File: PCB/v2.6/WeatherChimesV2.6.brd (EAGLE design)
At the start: 99.3 x 79 mm, 31 parts, among them U1 MS5803-02BA, X4 BQ24074

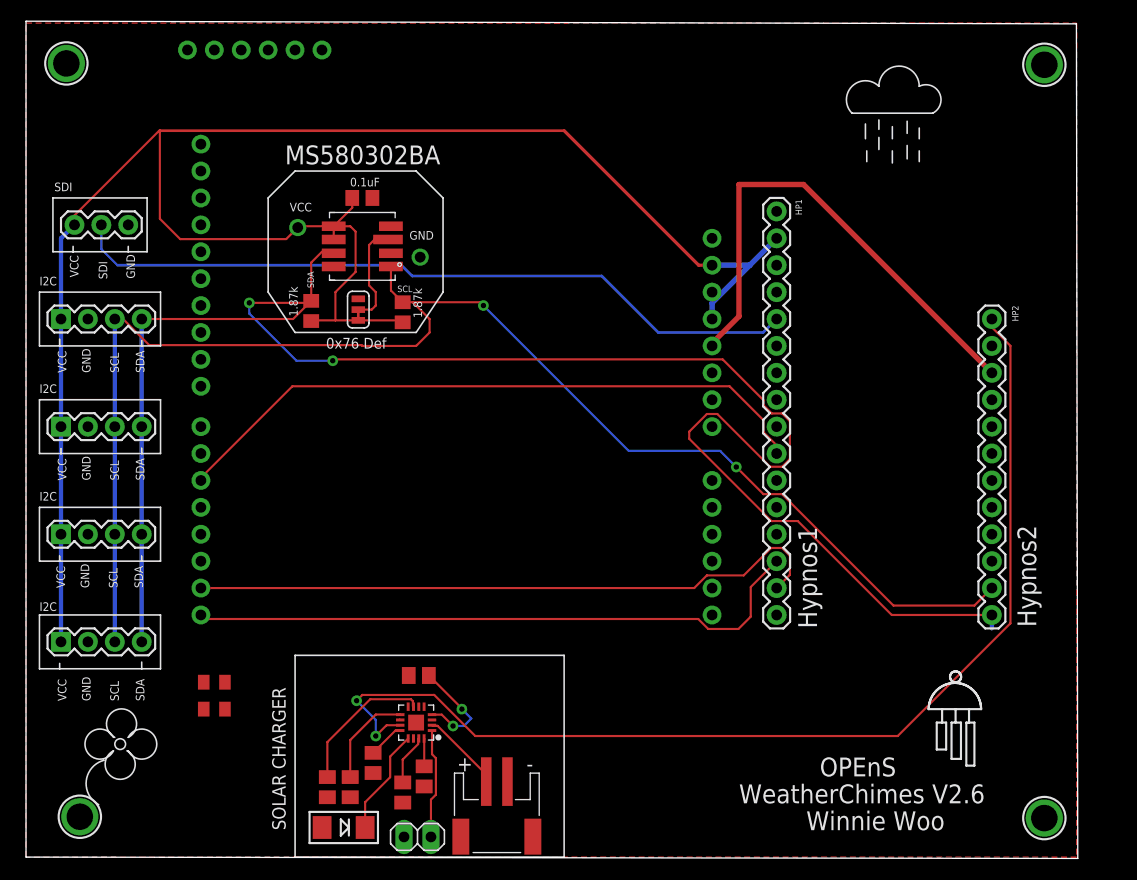
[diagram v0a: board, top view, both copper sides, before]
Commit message: WeatherChimesv2.6 files from Google Drive
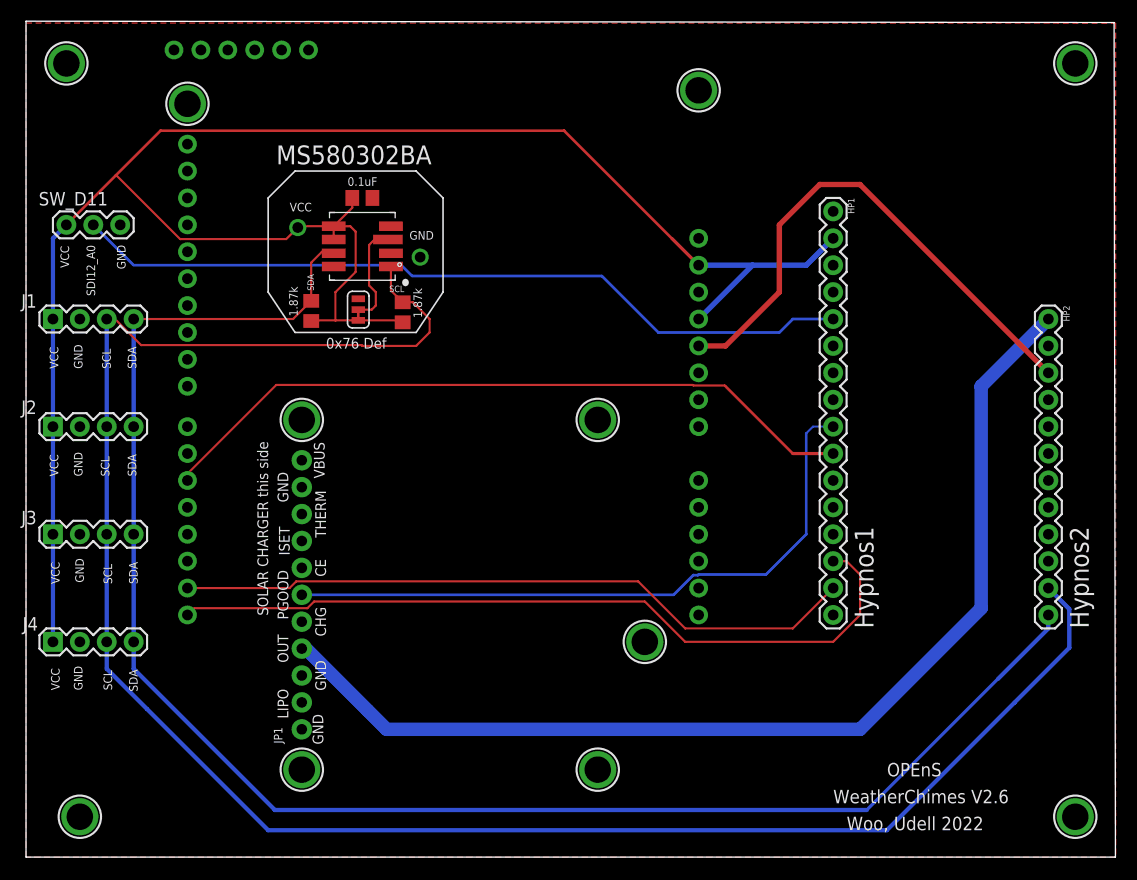
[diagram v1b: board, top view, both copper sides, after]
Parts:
- removed BATT: JST 2PH, adafruit:JST-PH-2-SMT-RA
- removed C5, C6: 10uF, adafruit:C0805K
- removed D2: SK34A, microbuilder:SMADIODE
- removed JP8: (no value), pinhead:1X02
- removed R11, R4, R7, R8: 10K, adafruit:M0805
- removed R3, R9: 1K, adafruit:M0805
- removed X4: BQ24074, adafruit_power:QFN16_3MM
- added JP1: (no value), microbuilder:1X11_ROUND_76
- added U$13, U$14, U$15, U$16, U$6, U$7, U$8: MOUNTINGHOLE2.5, microbuilder:MOUNTINGHOLE_2.5_PLATED
- moved HP1 5.33 mm to (74.9, 62.2)
- moved HP2 5.33 mm to (95.2, 52.1)
- moved U$4 2.92 mm to (97.8, 76.2)
- moved U$5 2.92 mm to (97.8, 5.08)
- moved U$1 1.27 mm to (62.2, 59.7)
- moved J1 0.76 mm to (1.27, 52.1)
- moved J2 0.76 mm to (1.27, 41.9)
- moved J3 0.76 mm to (1.27, 31.8)
- moved J4 0.76 mm to (1.27, 21.6)
- moved SW_D11 0.76 mm to (2.54, 61.0)
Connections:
- removed net !CE: R8.1, X4.4
- removed net !CHG: R7.1, X4.9
- removed net !PGOOD: R11.1, X4.7
- removed net CHARGER_IN: D2.A
- removed net ILIM: R3.1, X4.12
- removed net ISET: R9.1, X4.16
- removed net ITERM: R4.1, X4.15
- removed net N$1: X4.5
- removed net N$2: D2.C, X4.13
- removed net THERM: JP8.1, X4.1
- removed net VLIPO: BATT.1, X4.2, X4.3
- net GND: now also JP1.1, JP1.10, JP1.3; no longer BATT.2, JP8.2, R3.2, R4.2, R8.2, R9.2, X4.14, X4.6, X4.8, X4.THERMAL
- net PGOOD: now also JP1.6
- net VBAT: now also JP1.4; no longer X4.10, X4.11
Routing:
- net PGOOD: track 0.00 -> 62.3 mm
- net SCL: track 137.3 -> 184.2 mm, vias 2 -> 0
- net RX: track 58.7 -> 73.5 mm
- net !PGOOD: track 13.7 -> 0.00 mm
- net SDA: track 169.5 -> 157.0 mm, vias 2 -> 0
- net THERM: track 10.4 -> 0.00 mm
- net !CE: track 10.2 -> 0.00 mm, vias 2 -> 0
- net N$2: track 10.1 -> 0.00 mm
- net !CHG: track 9.76 -> 0.00 mm
- net VLIPO: track 7.72 -> 0.00 mm
- net 4GONOFF: track 62.7 -> 67.7 mm
- net ITERM: track 4.78 -> 0.00 mm
- net SDI: track 70.6 -> 74.6 mm
- net VCC: track 174.2 -> 177.9 mm
- net TX: track 61.0 -> 64.6 mm
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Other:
- board size 99.3 x 79 mm -> 102.8 x 78.9 mm
- board text added: "CE"
- board text added: "CHG"
- board text added: "ISET"
- board text added: "LIPO"
- board text added: "OUT"
- board text added: "PGOOD"
- board text added: "SDI12_A0"
- board text added: "SOLAR CHARGER this side"
- board text added: "THERM"
- board text added: "VBUS"
- board text added: "Woo, Udell 2022"
- board text added: "•"
- board text removed: "I2C"
- board text removed: "SDI"
- board text removed: "SOLAR CHARGER"
- board text removed: "Winnie Woo"
